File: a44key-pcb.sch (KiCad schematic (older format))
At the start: 68 parts, among them J1 AudioJack3, J2 Conn_01x04_Female, J3 Conn_01x04_Female, J4 Conn_01x04_Female, SW1 SW_Push, U1 ATmega32U4-AU, Y1 16MHz

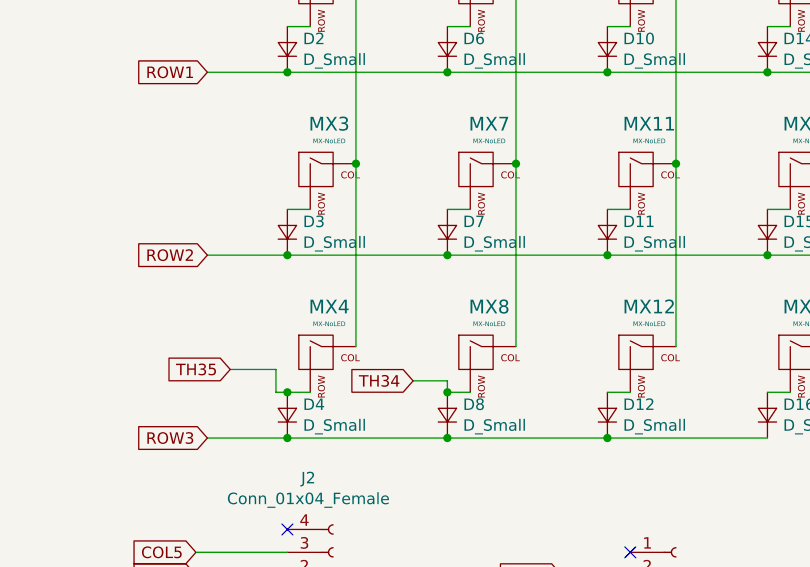
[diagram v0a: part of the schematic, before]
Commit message: {PCB
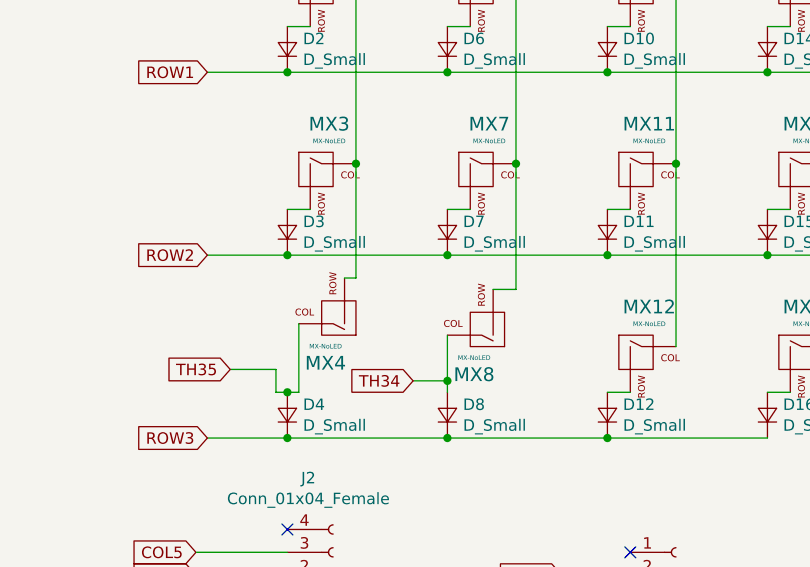
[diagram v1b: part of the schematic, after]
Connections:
- net COL4: now also MX8.2 (ROW); no longer MX8.1 (COL)
- net COL5: now also MX4.2 (ROW); no longer MX4.1 (COL)
- net TH34: now also MX8.1 (COL); no longer MX8.2 (ROW)
- net TH35: now also MX4.1 (COL); no longer MX4.2 (ROW)
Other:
- moved on the sheet: MX4, MX8
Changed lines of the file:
@@
 L MX_Alps_Hybrid:MX-NoLED MX4
 U 1 1 61713060
-P 6700 4750
-F 0 "MX4" H 6733 4973 60  0000 C CNN
-F 1 "MX-NoLED" H 6733 4899 20  0000 C CNN
-F 2 "MX_Alps_Hybrid:MX-Alps-Choc-X-1U-NoLED" H 6075 4725 60  0001 C CNN
-F 3 "" H 6075 4725 60  0001 C CNN
-	1    6700 4750
-	1    0    0    -1
+P 6750 4550
+F 0 "MX4" H 6783 4773 60  0000 C CNN
+F 1 "MX-NoLED" H 6783 4699 20  0000 C CNN
+F 2 "MX_Alps_Hybrid:MX-Alps-Choc-X-1U-NoLED" H 6125 4525 60  0001 C CNN
+F 3 "" H 6125 4525 60  0001 C CNN
+	1    6750 4550
+	-1   0    0    1
 $EndComp
 $Comp
@@
 $EndComp
 Wire Wire Line
-	6550 4900 6650 4900
+	6550 4900 6600 4900
 $Comp
 L MX_Alps_Hybrid:MX-NoLED MX8
 U 1 1 6171306D
-P 7400 4750
-F 0 "MX8" H 7433 4973 60  0000 C CNN
-F 1 "MX-NoLED" H 7433 4899 20  0000 C CNN
-F 2 "MX_Alps_Hybrid:MX-Alps-Choc-X-1U-NoLED" H 6775 4725 60  0001 C CNN
-F 3 "" H 6775 4725 60  0001 C CNN
-	1    7400 4750
-	1    0    0    -1
+P 7400 4600
+F 0 "MX8" H 7433 4823 60  0000 C CNN
+F 1 "MX-NoLED" H 7433 4749 20  0000 C CNN
+F 2 "MX_Alps_Hybrid:MX-Alps-Choc-X-1U-NoLED" H 6775 4575 60  0001 C CNN
+F 3 "" H 6775 4575 60  0001 C CNN
+	1    7400 4600
+	-1   0    0    1
 $EndComp
 $Comp
@@
 	0    -1   -1   0
 $EndComp
-Wire Wire Line
-	7250 4900 7350 4900
 $Comp
 L MX_Alps_Hybrid:MX-NoLED MX11
@@
 Connection ~ 6850 3100
 Wire Wire Line
-	6850 3900 6850 4700
-Connection ~ 6850 3900
-Wire Wire Line
 	7550 2300 7550 3100
 Wire Wire Line
 	7550 3100 7550 3900
 Connection ~ 7550 3100
-Wire Wire Line
-	7550 3900 7550 4700
-Connection ~ 7550 3900
 Wire Wire Line
 	8250 2300 8250 3100
@@
 Wire Wire Line
 	7250 4850 7250 4900
-Connection ~ 7250 4900
 $Comp
 L Device:C_Small C8
@@
 NoConn ~ 8100 6150
 NoConn ~ 8100 6450
+Wire Wire Line
+	6850 3900 6850 4400
+Wire Wire Line
+	6850 4400 6800 4400
+Connection ~ 6850 3900
+Wire Wire Line
+	6600 4600 6600 4900
+Wire Wire Line
+	7550 3900 7550 4450
+Wire Wire Line
+	7550 4450 7450 4450
+Connection ~ 7550 3900
+Wire Wire Line
+	7250 4650 7250 4850
+Connection ~ 7250 4850
 $EndSCHEMATC

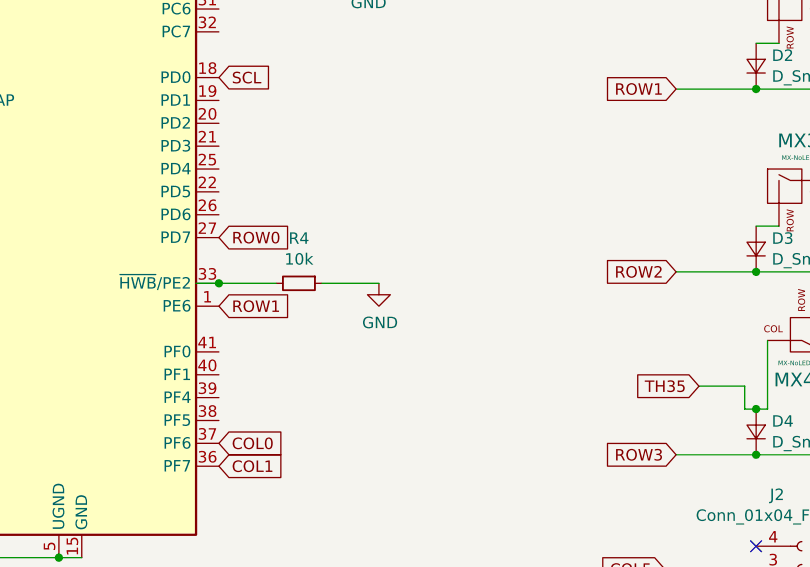
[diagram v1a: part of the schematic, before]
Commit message: PCB
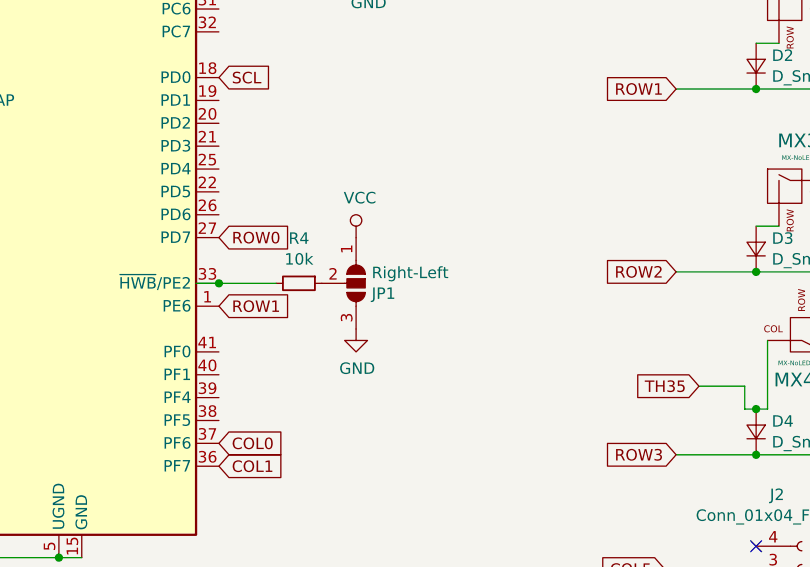
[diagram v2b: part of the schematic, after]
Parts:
- added Right-Left: JP1, Jumper:SolderJumper-3_P1.3mm_Open_Pad1.0x1.5mm, symbol Jumper:SolderJumper_3_Open
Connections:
- net GND: now also Right-Left.3 (B); no longer R4.1
- net VCC: now also Right-Left.1 (A)
- new net: R4.1, Right-Left.2 (C)
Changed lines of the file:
@@
 L power:GND #PWR0103
 U 1 1 616B6C85
-P 4900 4350
-F 0 "#PWR0103" H 4900 4100 50  0001 C CNN
-F 1 "GND" H 4905 4177 50  0000 C CNN
-F 2 "" H 4900 4350 50  0001 C CNN
-F 3 "" H 4900 4350 50  0001 C CNN
-	1    4900 4350
-	1    0    0    -1
-$EndComp
-Wire Wire Line
-	4900 4350 4650 4350
+P 4800 4550
+F 0 "#PWR0103" H 4800 4300 50  0001 C CNN
+F 1 "GND" H 4805 4377 50  0000 C CNN
+F 2 "" H 4800 4550 50  0001 C CNN
+F 3 "" H 4800 4550 50  0001 C CNN
+	1    4800 4550
+	1    0    0    -1
+$EndComp
 Connection ~ 4200 4350
 Wire Wire Line
@@
 	7250 4650 7250 4850
 Connection ~ 7250 4850
+$Comp
+L power:VCC #PWR0123
+U 1 1 61D90AAA
+P 4800 4150
+F 0 "#PWR0123" H 4800 4000 50  0001 C CNN
+F 1 "VCC" H 4817 4323 50  0000 C CNN
+F 2 "" H 4800 4150 50  0001 C CNN
+F 3 "" H 4800 4150 50  0001 C CNN
+	1    4800 4150
+	1    0    0    -1
+$EndComp
+$Comp
+L Jumper:SolderJumper_3_Open Right-Left
+U 1 1 61D817AC
+P 4800 4350
+F 0 "Right-Left" V 4754 4418 50  0000 L CNN
+F 1 "JP1" V 4845 4418 50  0000 L CNN
+F 2 "Jumper:SolderJumper-3_P1.3mm_Open_Pad1.0x1.5mm" H 4800 4350 50  0001 C CNN
+F 3 "~" H 4800 4350 50  0001 C CNN
+	1    4800 4350
+	0    1    1    0
+$EndComp
 $EndSCHEMATC
